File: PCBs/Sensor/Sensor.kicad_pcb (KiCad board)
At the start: 2 copper layers, 35 x 45 mm, 9 parts, among them J1 RJ45, J2 RJ45, J3 Conn_01x04_Pin, U1 ATtiny85-20P

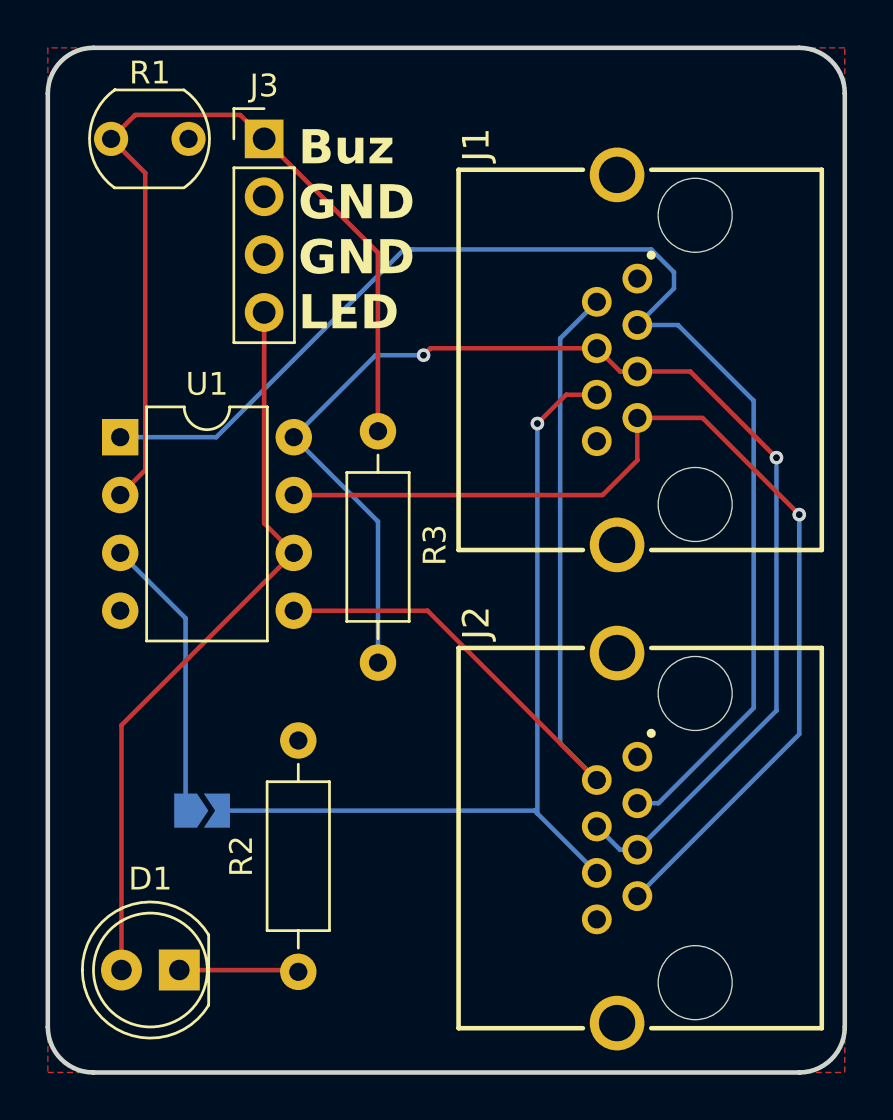
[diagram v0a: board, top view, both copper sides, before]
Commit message: update sensor
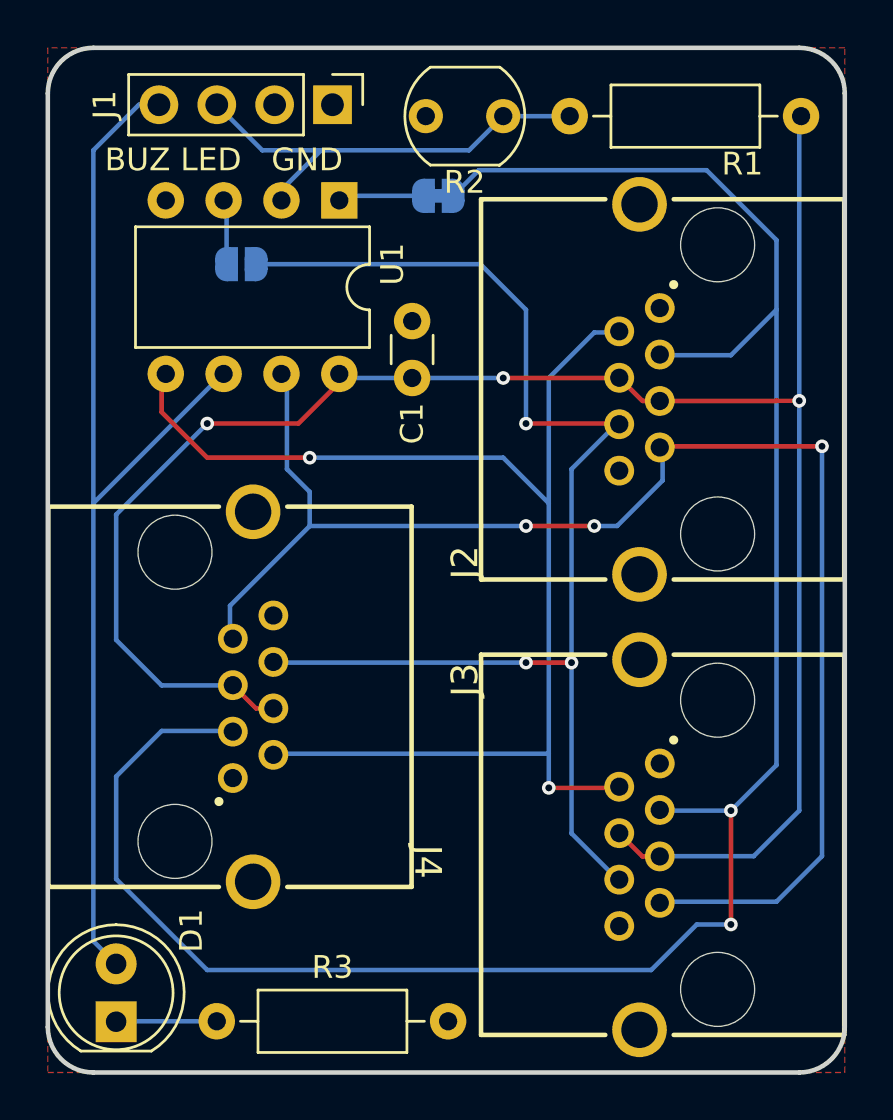
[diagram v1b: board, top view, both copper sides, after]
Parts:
- added C1: 0.1μ, Capacitor_THT:C_Disc_D3.0mm_W1.6mm_P2.50mm, F.Cu at (66.0, 64.5)
- added J4: RJ45, Library:WR-MJ Modular Jack Horizontal Shielded w. EMI Panel Finger 8P8C Tab Up, F.Cu at (58.0, 78.5)
- added JP2: Jumper_2_Open, Jumper:SolderJumper-2_P1.3mm_Open_RoundedPad1.0x1.5mm, B.Cu at (58.5, 59.5)
- J1: value RJ45 -> Conn_01x04_Pin; footprint Library:WR-MJ Modular Jack Horizontal Shielded w. EMI Panel Finger 8P8C Tab Up -> Connector_PinHeader_2.54mm:PinHeader_1x04_P2.54mm_Vertical
- J3: value Conn_01x04_Pin -> RJ45; footprint Connector_PinHeader_2.54mm:PinHeader_1x04_P2.54mm_Vertical -> Library:WR-MJ Modular Jack Horizontal Shielded w. EMI Panel Finger 8P8C Tab Up
- JP1: value Jumper_2_Open -> Jumper_2_Bridged; footprint Jumper:SolderJumper-2_P1.3mm_Open_TrianglePad1.0x1.5mm -> Jumper:SolderJumper-2_P1.3mm_Bridged_RoundedPad1.0x1.5mm
- R1: value LDR07 -> 10k; footprint OptoDevice:R_LDR_5.1x4.3mm_P3.4mm_Vertical -> Resistor_THT:R_Axial_DIN0207_L6.3mm_D2.5mm_P10.16mm_Horizontal
- R2: value 220 -> LDR07; footprint Resistor_THT:R_Axial_DIN0207_L6.3mm_D2.5mm_P10.16mm_Horizontal -> OptoDevice:R_LDR_5.1x4.3mm_P3.4mm_Vertical
- R3: value 10k -> 220
- moved J3 35.6 mm to (77.0, 85.0), turned to 90 degrees
- moved JP1 28.9 mm to (67.2, 56.5)
- moved R2 28.9 mm to (70.0, 53.0), turned to 180 degrees
- moved R1 20.2 mm to (72.9, 53.0)
- moved J2 19.7 mm to (77.0, 65.0)
- moved J1 17.6 mm to (62.5, 52.5), turned to -90 degrees
- moved R3 17.3 mm to (57.4, 92.8), turned to 0 degrees
- moved U1 14.2 mm to (62.8, 56.7), turned to -90 degrees
- moved D1 3.59 mm to (53.0, 92.8), turned to 90 degrees
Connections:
- J1 pad 2: /SDA -> GND
- J1 pad 3: /Reset -> /in
- J1 pad 4: +5V -> /out
- J2 pad 2: /SDA -> /SDA0
- J2 pad 3: /Reset -> Net-(JP1-B)
- J2 pad 4: +5V -> +3.3V
- J2 pad 5: +5V -> +3.3V
- J2 pad 6: Net-(JP1-B) -> Net-(JP2-B)
- J2 pad 7: /SCL -> /SCL0
- J3 pad 1: /in -> GND
- J3 pad 2: GND -> /SDA0
- J3 pad 3: GND -> Net-(JP1-B)
- J3 pad 4: /out -> +3.3V
- JP1 pad 1: Net-(JP1-A) -> /AT_RS
- R1 pad 2: GND -> +3.3V
- R2 pad 1: GND -> /in
- R2 pad 2: Net-(D1-K) -> GND
- R3 pad 1: +5V -> Net-(D1-K)
- R3 pad 2: /in -> GND
- U1 pad 1: /Reset -> /AT_RS
- U1 pad 3: Net-(JP1-A) -> /FU
- U1 pad 5: /SDA -> /SDA0
- U1 pad 7: /SCL -> /SCL0
- U1 pad 8: +5V -> +3.3V
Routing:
- net +3.3V: track 0.00 -> 86.9 mm, vias 0 -> 3
- net /SCL0: track 0.00 -> 64.6 mm, vias 0 -> 3
- net /Reset: track 58.0 -> 0.00 mm
- net Net-(JP1-B): track 38.0 -> 95.9 mm, vias 1 -> 2
- net +5V: track 57.8 -> 0.00 mm, vias 2 -> 0
- net /SDA0: track 0.00 -> 57.6 mm, vias 0 -> 2
- net Net-(JP2-B): track 0.00 -> 56.8 mm, vias 0 -> 3
- net /SCL: track 46.1 -> 0.00 mm, vias 1 -> 0
- net /SDA: track 39.1 -> 0.00 mm
- net /in: track 39.2 -> 19.9 mm
- net /out: track 32.6 -> 47.9 mm
- net Net-(JP1-A): track 12.5 -> 0.00 mm
- net /AT_RS: track 0.00 -> 3.78 mm
- net /FU: track 0.00 -> 2.85 mm
- net Net-(D1-K): track 5.26 -> 4.43 mm
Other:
- board text added: "BUZ LED GND"
- board text removed: "Buz GND GND LED"
